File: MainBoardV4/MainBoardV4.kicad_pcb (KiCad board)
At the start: 2 copper layers, 100 x 100 mm, 85 parts, among them J1 Conn_01x02, J11 Conn_01x03, J12 USB_B_Micro, J13 Conn_02x03_Odd_Even, J14 Conn_01x04, J15 Conn_02x03_Odd_Even, J16 Conn_01x04, J17 Conn_02x03_Odd_Even, J18 Conn_01x04, J19 Conn_01x04, J2 Conn_01x02, J20 Conn_01x04, J21 Conn_01x04, J22 Conn_01x05, J23 Conn_02x05_Odd_Even, J24 Conn_01x03, J25 Conn_01x05, J3 Conn_01x02, J5 Conn_01x02, J6 Conn_01x02, J7 Conn_01x02, J8 Conn_01x02, J9 Conn_01x02, SW1 SW_Push, U1 ESP32-S3-WROOM-1, U2 TSR_2-2433, U3 TSR_2-2450, U4 TEN_50-2411WI, U5 PCA9685PW, U6 Servo_Conn_Pack_x04, U7 Servo_Conn_Pack_x04, U8 Servo_Conn_Pack_x04, U9 Servo_Conn_Pack_x04

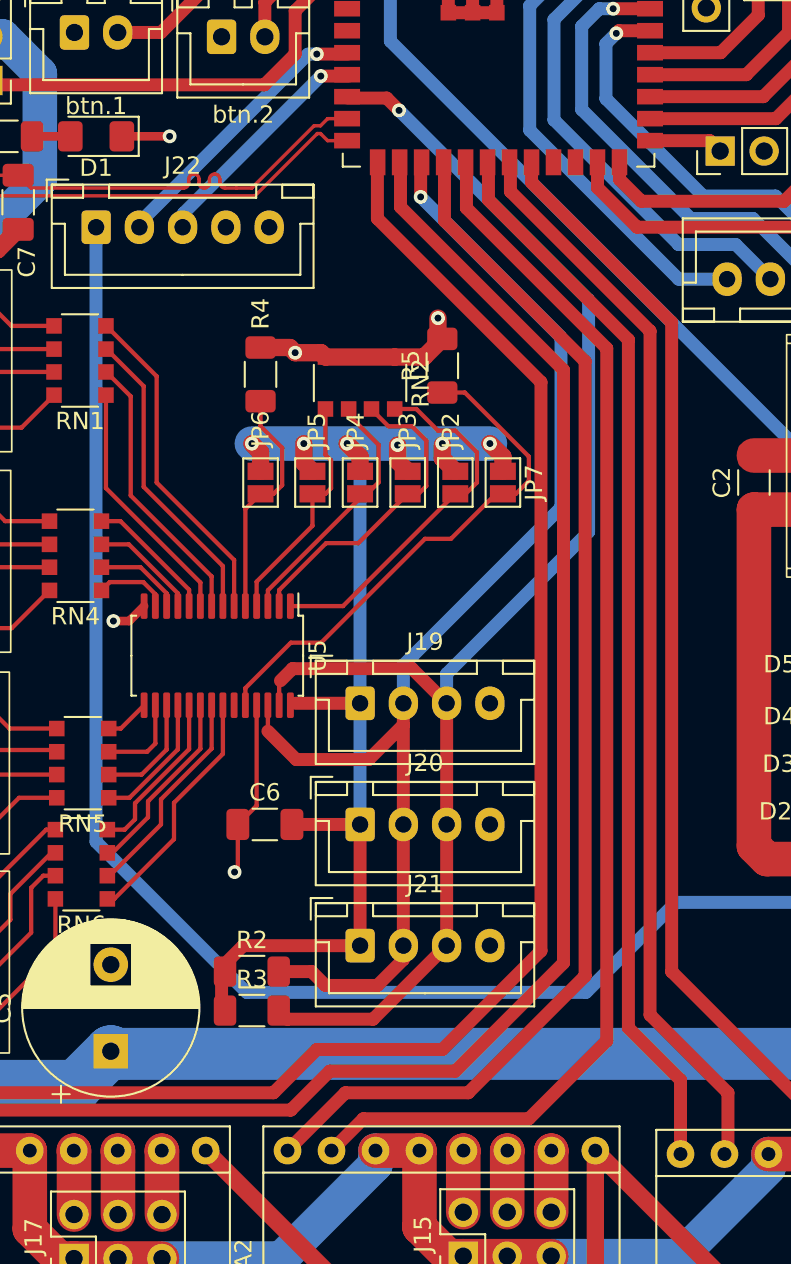
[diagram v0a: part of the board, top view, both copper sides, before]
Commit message: test
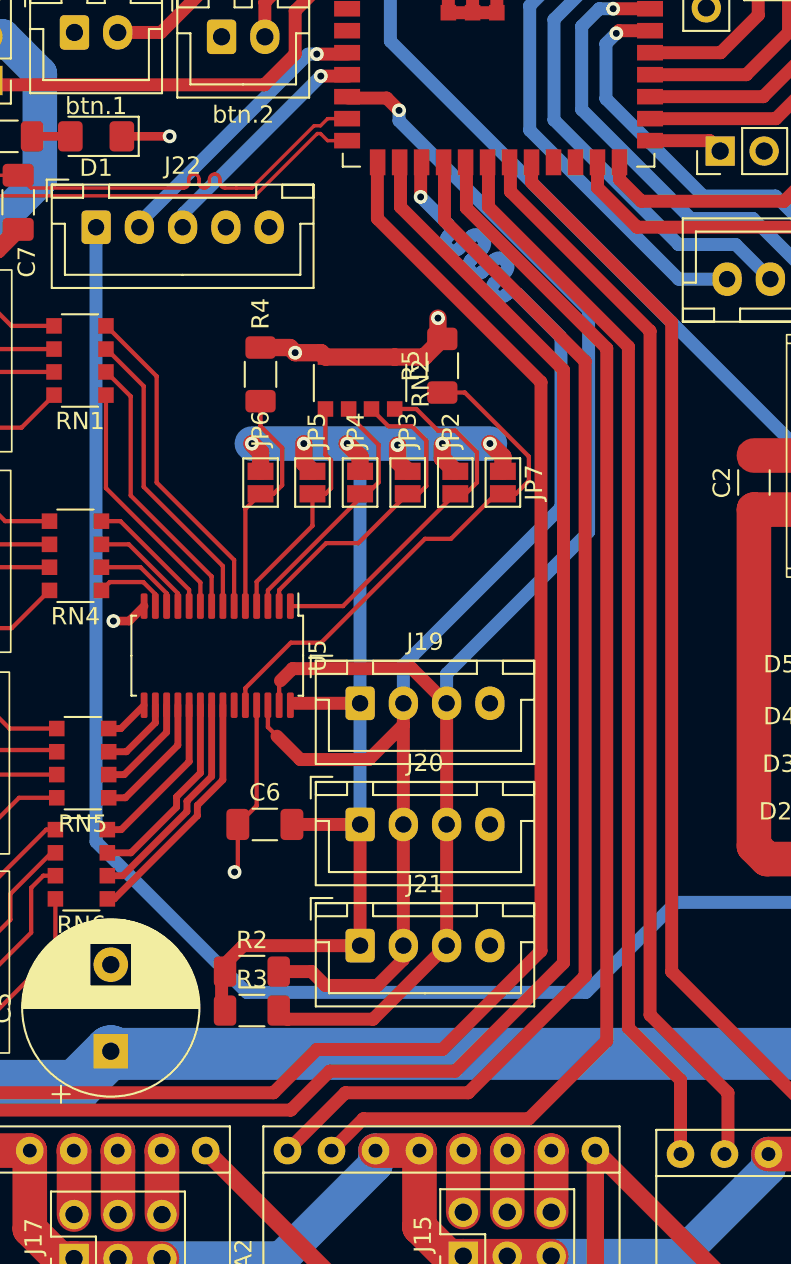
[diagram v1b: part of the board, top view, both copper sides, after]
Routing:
- net SCL: track 73.4 -> 80.1 mm
- net Net-(RN5-R3.1): track 5.10 -> 4.40 mm
- net Net-(RN6-R3.1): track 10.9 -> 11.6 mm
- net Net-(RN5-R2.1): track 6.51 -> 5.92 mm
